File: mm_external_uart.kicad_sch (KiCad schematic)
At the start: 1 part, among them J4 Conn_01x04_Pin

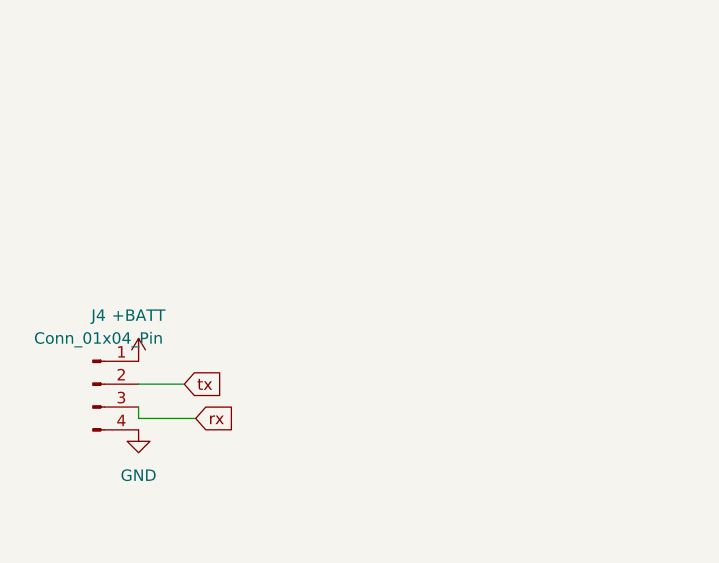
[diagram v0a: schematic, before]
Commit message: TP3
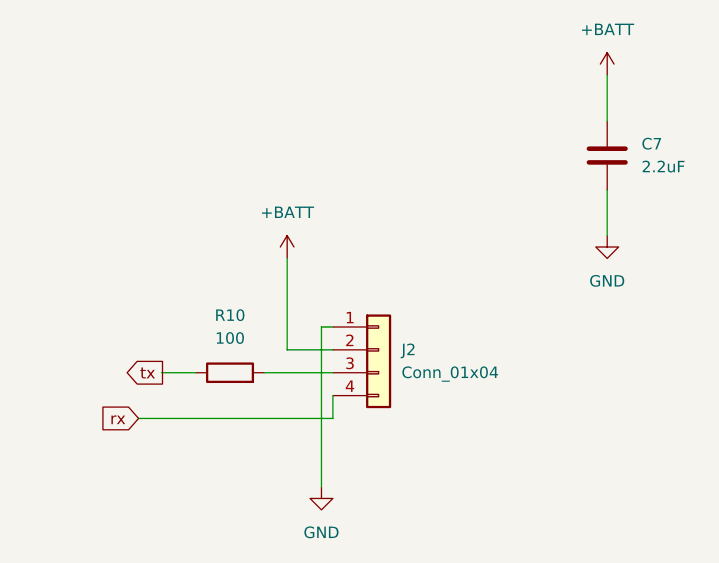
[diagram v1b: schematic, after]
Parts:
- removed J4: Conn_01x04_Pin, symbol Connector:Conn_01x04_Pin
- added C7: 2.2uF, Capacitor_SMD:C_0603_1608Metric, symbol Device:C
- added J2: Conn_01x04, Connector_PinHeader_2.54mm:PinHeader_1x04_P2.54mm_Vertical, symbol Connector_Generic:Conn_01x04
- added R10: 100, Resistor_SMD:R_0603_1608Metric, symbol Device:R
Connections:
- net +BATT: now also C7.1, J2.2 (Pin_2)
- net GND: now also C7.2, J2.1 (Pin_1)
- net rx: now also J2.4 (Pin_4)
- new net: J2.3 (Pin_3), R10.2
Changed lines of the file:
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@@
 (kicad_sch (version 20230121) (generator eeschema)
   (paper "A4")
-  (wire (pts (xy 77.47 80.01) (xy 82.55 80.01))
-    (stroke (width 0) (type default))
-  )
-  (wire (pts (xy 77.47 83.82) (xy 83.82 83.82))
-    (stroke (width 0) (type default))
-  )
-  (wire (pts (xy 77.47 82.55) (xy 77.47 83.82))
-    (stroke (width 0) (type default))
-  )
-  (global_label "tx" (shape input) (at 82.55 80.01 0) (fields_autoplaced)
+  (wire (pts (xy 93.98 66.04) (xy 93.98 76.2))
+    (stroke (width 0) (type default))
+  )
+  (wire (pts (xy 80.01 78.74) (xy 83.82 78.74))
+    (stroke (width 0) (type default))
+  )
+  (wire (pts (xy 129.54 58.42) (xy 129.54 63.5))
+    (stroke (width 0) (type default))
+  )
+  (wire (pts (xy 99.06 83.82) (xy 99.06 81.28))
+    (stroke (width 0) (type default))
+  )
+  (wire (pts (xy 77.47 83.82) (xy 99.06 83.82))
+    (stroke (width 0) (type default))
+  )
+  (wire (pts (xy 97.79 73.66) (xy 97.79 91.44))
+    (stroke (width 0) (type default))
+  )
+  (wire (pts (xy 91.44 78.74) (xy 99.06 78.74))
+    (stroke (width 0) (type default))
+  )
+  (wire (pts (xy 99.06 76.2) (xy 93.98 76.2))
+    (stroke (width 0) (type default))
+  )
+  (wire (pts (xy 129.54 45.72) (xy 129.54 50.8))
+    (stroke (width 0) (type default))
+  )
+  (wire (pts (xy 99.06 73.66) (xy 97.79 73.66))
+    (stroke (width 0) (type default))
+  )
+  (global_label "tx" (shape input) (at 76.2 78.74 0) (fields_autoplaced)
     (effects (font (size 1.27 1.27)) (justify left))
-    (property "Intersheetrefs" "${INTERSHEET_REFS}" (at 87.289 80.01 0)
+    (property "Intersheetrefs" "${INTERSHEET_REFS}" (at 80.939 78.74 0)
       (effects (font (size 1.27 1.27)) (justify left) hide)
     )
   )
-  (global_label "rx" (shape input) (at 83.82 83.82 0) (fields_autoplaced)
-    (effects (font (size 1.27 1.27)) (justify left))
-    (property "Intersheetrefs" "${INTERSHEET_REFS}" (at 88.6195 83.82 0)
-      (effects (font (size 1.27 1.27)) (justify left) hide)
-    )
-  )
-  (symbol (lib_id "power:GND") (at 77.47 85.09 0) (unit 1)
-    (in_bom yes) (on_board yes) (dnp no) (fields_autoplaced)
-    (property "Reference" "#PWR08" (at 77.47 91.44 0)
-      (effects (font (size 1.27 1.27)) hide)
-    )
-    (property "Value" "GND" (at 77.47 90.17 0)
-      (effects (font (size 1.27 1.27)))
-    )
-    (property "Footprint" "" (at 77.47 85.09 0)
-      (effects (font (size 1.27 1.27)) hide)
-    )
-    (property "Datasheet" "" (at 77.47 85.09 0)
-      (effects (font (size 1.27 1.27)) hide)
-    )
-    (pin "1")
-    (instances
-      (project "minimouse"
+  (global_label "rx" (shape input) (at 77.47 83.82 180) (fields_autoplaced)
+    (effects (font (size 1.27 1.27)) (justify right))
+    (property "Intersheetrefs" "${INTERSHEET_REFS}" (at 72.6705 83.82 0)
+      (effects (font (size 1.27 1.27)) (justify right) hide)
+    )
+  )
+  (symbol (lib_id "power:GND") (at 97.79 91.44 0) (unit 1)
+    (in_bom yes) (on_board yes) (dnp no) (fields_autoplaced)
+    (property "Reference" "#PWR08" (at 97.79 97.79 0)
+      (effects (font (size 1.27 1.27)) hide)
+    )
+    (property "Value" "GND" (at 97.79 96.52 0)
+      (effects (font (size 1.27 1.27)))
+    )
+    (property "Footprint" "" (at 97.79 91.44 0)
+      (effects (font (size 1.27 1.27)) hide)
+    )
+    (property "Datasheet" "" (at 97.79 91.44 0)
+      (effects (font (size 1.27 1.27)) hide)
+    )
+    (pin "1")
+    (instances
+      (project "tp2cao"
         (path "/d8fa4cba-2469-4231-847f-065b6b829f44/d17bb1c7-f68a-465e-9a17-5858ef86fc30"
           (reference "#PWR08") (unit 1)
@@
     )
   )
-  (symbol (lib_id "Connector:Conn_01x04_Pin") (at 72.39 80.01 0) (unit 1)
-    (in_bom yes) (on_board yes) (dnp no) (fields_autoplaced)
-    (property "Reference" "J4" (at 73.025 72.39 0)
-      (effects (font (size 1.27 1.27)))
-    )
-    (property "Value" "Conn_01x04_Pin" (at 73.025 74.93 0)
-      (effects (font (size 1.27 1.27)))
-    )
-    (property "Footprint" "" (at 72.39 80.01 0)
-      (effects (font (size 1.27 1.27)) hide)
-    )
-    (property "Datasheet" "~" (at 72.39 80.01 0)
-      (effects (font (size 1.27 1.27)) hide)
-    )
-    (pin "1")
+  (symbol (lib_id "Device:R") (at 87.63 78.74 90) (unit 1)
+    (in_bom yes) (on_board yes) (dnp no) (fields_autoplaced)
+    (property "Reference" "R10" (at 87.63 72.39 90)
+      (effects (font (size 1.27 1.27)))
+    )
+    (property "Value" "100" (at 87.63 74.93 90)
+      (effects (font (size 1.27 1.27)))
+    )
+    (property "Footprint" "Resistor_SMD:R_0603_1608Metric" (at 87.63 80.518 90)
+      (effects (font (size 1.27 1.27)) hide)
+    )
+    (property "Datasheet" "~" (at 87.63 78.74 0)
+      (effects (font (size 1.27 1.27)) hide)
+    )
     (pin "2")
+    (pin "1")
+    (instances
+      (project "tp2cao"
+        (path "/d8fa4cba-2469-4231-847f-065b6b829f44/d17bb1c7-f68a-465e-9a17-5858ef86fc30"
+          (reference "R10") (unit 1)
+        )
+      )
+    )
+  )
+  (symbol (lib_id "power:+BATT") (at 93.98 66.04 0) (unit 1)
+    (in_bom yes) (on_board yes) (dnp no) (fields_autoplaced)
+    (property "Reference" "#PWR032" (at 93.98 69.85 0)
+      (effects (font (size 1.27 1.27)) hide)
+    )
+    (property "Value" "+BATT" (at 93.98 60.96 0)
+      (effects (font (size 1.27 1.27)))
+    )
+    (property "Footprint" "" (at 93.98 66.04 0)
+      (effects (font (size 1.27 1.27)) hide)
+    )
+    (property "Datasheet" "" (at 93.98 66.04 0)
+      (effects (font (size 1.27 1.27)) hide)
+    )
+    (pin "1")
+    (instances
+      (project "tp2cao"
+        (path "/d8fa4cba-2469-4231-847f-065b6b829f44/d17bb1c7-f68a-465e-9a17-5858ef86fc30"
+          (reference "#PWR032") (unit 1)
+        )
+      )
+    )
+  )
+  (symbol (lib_id "power:GND") (at 129.54 63.5 0) (unit 1)
+    (in_bom yes) (on_board yes) (dnp no) (fields_autoplaced)
+    (property "Reference" "#PWR033" (at 129.54 69.85 0)
+      (effects (font (size 1.27 1.27)) hide)
+    )
+    (property "Value" "GND" (at 129.54 68.58 0)
+      (effects (font (size 1.27 1.27)))
+    )
+    (property "Footprint" "" (at 129.54 63.5 0)
+      (effects (font (size 1.27 1.27)) hide)
+    )
+    (property "Datasheet" "" (at 129.54 63.5 0)
+      (effects (font (size 1.27 1.27)) hide)
+    )
+    (pin "1")
+    (instances
+      (project "tp2cao"
+        (path "/d8fa4cba-2469-4231-847f-065b6b829f44/d17bb1c7-f68a-465e-9a17-5858ef86fc30"
+          (reference "#PWR033") (unit 1)
+        )
+      )
+    )
+  )
+  (symbol (lib_id "power:+BATT") (at 129.54 45.72 0) (unit 1)
+    (in_bom yes) (on_board yes) (dnp no) (fields_autoplaced)
+    (property "Reference" "#PWR034" (at 129.54 49.53 0)
+      (effects (font (size 1.27 1.27)) hide)
+    )
+    (property "Value" "+BATT" (at 129.54 40.64 0)
+      (effects (font (size 1.27 1.27)))
+    )
+    (property "Footprint" "" (at 129.54 45.72 0)
+      (effects (font (size 1.27 1.27)) hide)
+    )
+    (property "Datasheet" "" (at 129.54 45.72 0)
+      (effects (font (size 1.27 1.27)) hide)
+    )
+    (pin "1")
+    (instances
+      (project "tp2cao"
+        (path "/d8fa4cba-2469-4231-847f-065b6b829f44/d17bb1c7-f68a-465e-9a17-5858ef86fc30"
+          (reference "#PWR034") (unit 1)
+        )
+      )
+    )
+  )
+  (symbol (lib_id "Device:C") (at 129.54 54.61 0) (unit 1)
+    (in_bom yes) (on_board yes) (dnp no) (fields_autoplaced)
+    (property "Reference" "C7" (at 133.35 53.34 0)
+      (effects (font (size 1.27 1.27)) (justify left))
+    )
+    (property "Value" "2.2uF" (at 133.35 55.88 0)
+      (effects (font (size 1.27 1.27)) (justify left))
+    )
+    (property "Footprint" "Capacitor_SMD:C_0603_1608Metric" (at 130.5052 58.42 0)
+      (effects (font (size 1.27 1.27)) hide)
+    )
+    (property "Datasheet" "~" (at 129.54 54.61 0)
+      (effects (font (size 1.27 1.27)) hide)
+    )
+    (pin "1")
+    (pin "2")
+    (instances
+      (project "tp2cao"
+        (path "/d8fa4cba-2469-4231-847f-065b6b829f44/d17bb1c7-f68a-465e-9a17-5858ef86fc30"
+          (reference "C7") (unit 1)
+        )
+      )
+    )
+  )
+  (symbol (lib_id "Connector_Generic:Conn_01x04") (at 104.14 76.2 0) (unit 1)
+    (in_bom yes) (on_board yes) (dnp no) (fields_autoplaced)
+    (property "Reference" "J2" (at 106.68 76.2 0)
+      (effects (font (size 1.27 1.27)) (justify left))
+    )
+    (property "Value" "Conn_01x04" (at 106.68 78.74 0)
+      (effects (font (size 1.27 1.27)) (justify left))
+    )
+    (property "Footprint" "Connector_PinHeader_2.54mm:PinHeader_1x04_P2.54mm_Vertical" (at 104.14 76.2 0)
+      (effects (font (size 1.27 1.27)) hide)
+    )
+    (property "Datasheet" "~" (at 104.14 76.2 0)
+      (effects (font (size 1.27 1.27)) hide)
+    )
+    (pin "2")
+    (pin "4")
+    (pin "1")
     (pin "3")
-    (pin "4")
-    (instances
-      (project "minimouse"
-        (path "/d8fa4cba-2469-4231-847f-065b6b829f44/d17bb1c7-f68a-465e-9a17-5858ef86fc30"
-          (reference "J4") (unit 1)
-        )
-      )
-    )
-  )
-  (symbol (lib_id "power:+BATT") (at 77.47 77.47 0) (unit 1)
-    (in_bom yes) (on_board yes) (dnp no) (fields_autoplaced)
-    (property "Reference" "#PWR013" (at 77.47 81.28 0)
-      (effects (font (size 1.27 1.27)) hide)
-    )
-    (property "Value" "+BATT" (at 77.47 72.39 0)
-      (effects (font (size 1.27 1.27)))
-    )
-    (property "Footprint" "" (at 77.47 77.47 0)
-      (effects (font (size 1.27 1.27)) hide)
-    )
-    (property "Datasheet" "" (at 77.47 77.47 0)
-      (effects (font (size 1.27 1.27)) hide)
-    )
-    (pin "1")
-    (instances
-      (project "minimouse"
-        (path "/d8fa4cba-2469-4231-847f-065b6b829f44/d17bb1c7-f68a-465e-9a17-5858ef86fc30"
-          (reference "#PWR013") (unit 1)
-        )
-      )
+    (instances
+      (project "tp2cao"
+        (path "/d8fa4cba-2469-4231-847f-065b6b829f44/d17bb1c7-f68a-465e-9a17-5858ef86fc30"
+          (reference "J2") (unit 1)
+        )
+      )
